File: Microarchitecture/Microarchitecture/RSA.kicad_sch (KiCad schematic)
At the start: 0 parts

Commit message: Added comments, 16 to 8 stage pipeline
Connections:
- no-connect marks 0 -> 1
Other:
- sheet AXI_RECEIVE_MODULE renamed AXI_IN
- sheet AXI_TRANSMIT_MODULE renamed AXI_OUT
- removed sheet RSA_STAGE_MODULE
- added sheet RSA_STAGE_MODULE3 (STAGE.kicad_sch)
- added sheet RSA_STAGE_MODULE8 (STAGE.kicad_sch)
- sheet AXI_IN ports: added ILO, IPI, MSGIN_LAST, MSGIN_READY, MSGIN_VALID; removed none
- sheet AXI_OUT ports: added IPI, IPO, MSGOUT_LAST, MSGOUT_READY, MSGOUT_VALID; removed none
- sheet RSA_STAGE_MODULE1 ports: added CS; removed none
- sheet RSA_STAGE_MODULE2 ports: added CS; removed none
- note added: "rsa_msgin"
- note added: "rsa_msgout"
- note added: "rsa_regio"

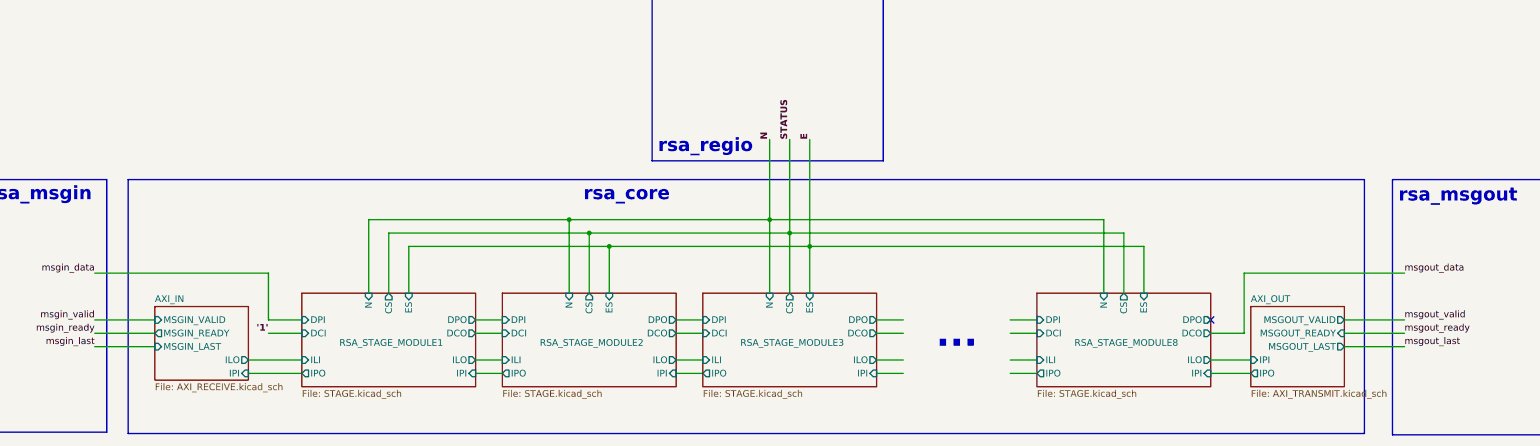
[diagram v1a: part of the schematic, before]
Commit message: Tried to update tb
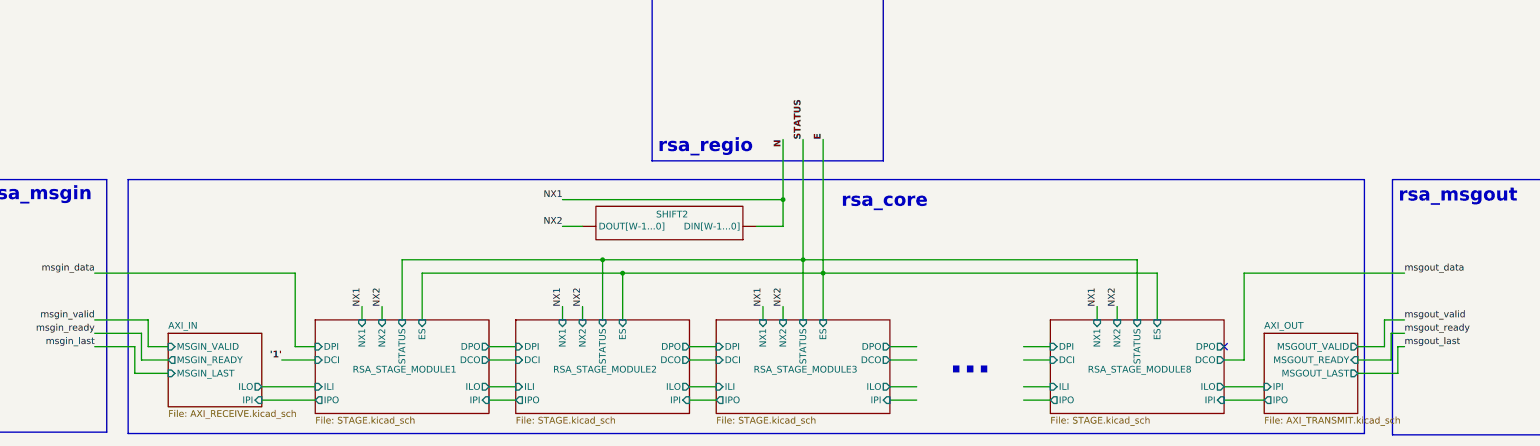
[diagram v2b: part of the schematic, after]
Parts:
- added SHIFT2: ~, symbol Symbols:SHIFT
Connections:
- net N: now also SHIFT2. (DOUT[W-1...0])
- new net NX2: SHIFT2. (DOUT[W-1...0])
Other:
- sheet RSA_STAGE_MODULE1 ports: added NX1, NX2, STATUS; removed CS, N
- sheet RSA_STAGE_MODULE2 ports: added NX1, NX2, STATUS; removed CS, N
- sheet RSA_STAGE_MODULE3 ports: added NX1, NX2, STATUS; removed CS, N
- sheet RSA_STAGE_MODULE8 ports: added NX1, NX2, STATUS; removed CS, N
